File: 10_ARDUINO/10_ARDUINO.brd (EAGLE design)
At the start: 67.4 x 44.8 mm, 3 parts, among them M1 ARDUINO_PROMINI, X1 ALLSERIALSLAVE

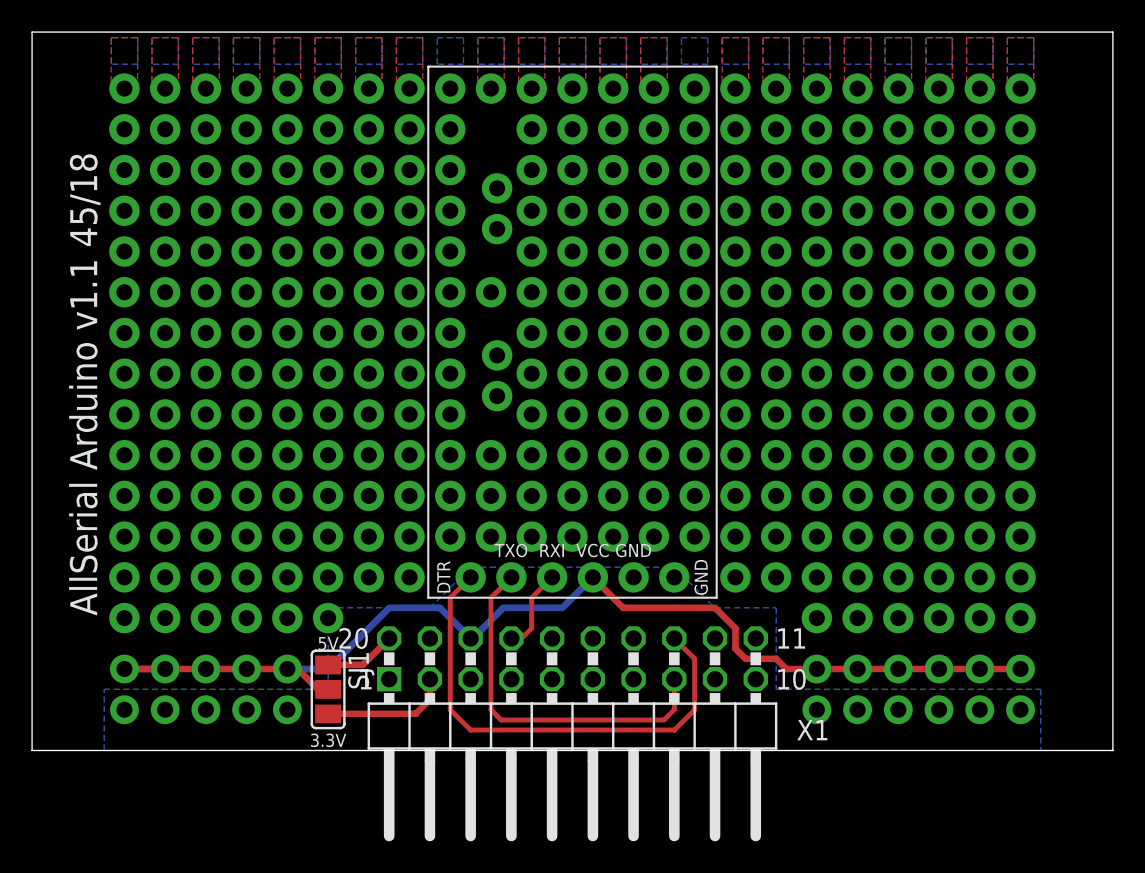
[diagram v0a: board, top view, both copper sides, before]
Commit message: Revert "pro mini layout corrected"
This reverts commit e6acf7b114fc184efa746b3a51c54623d1353390.
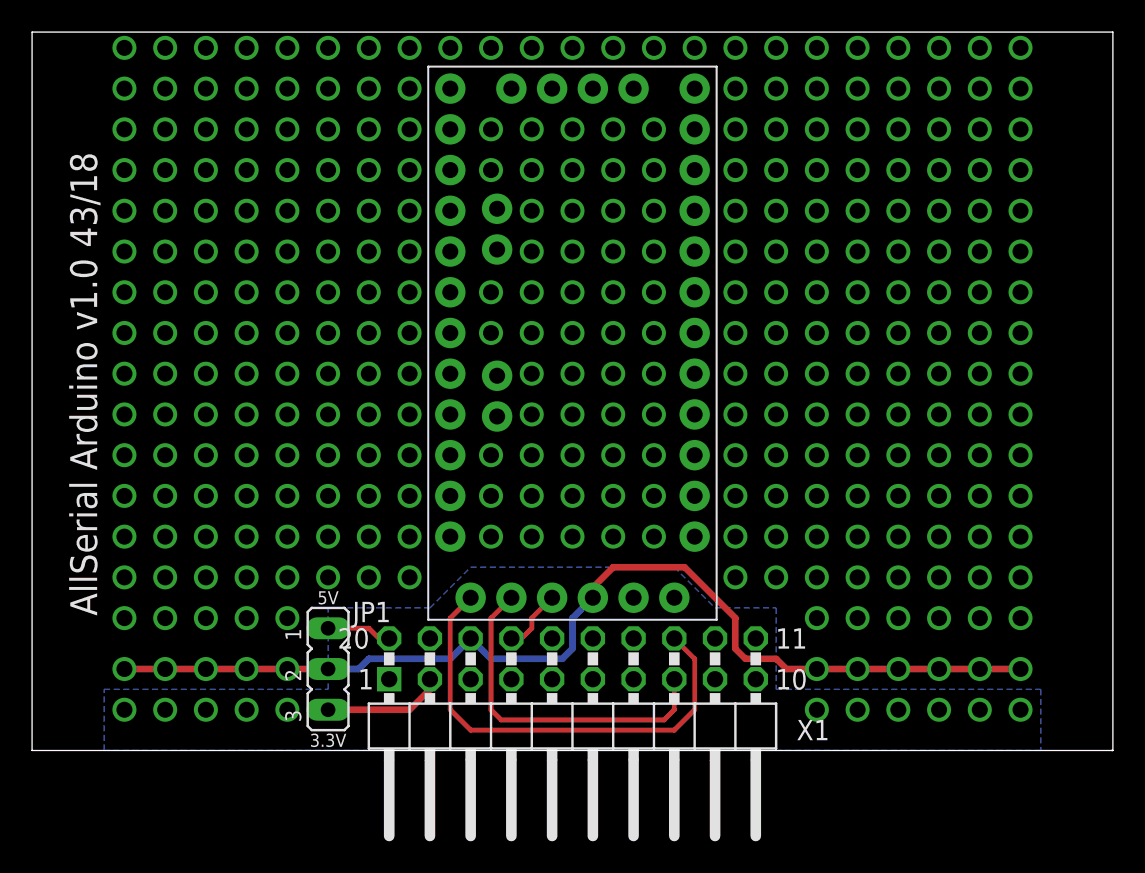
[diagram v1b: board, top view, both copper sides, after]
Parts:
- removed SJ1: (no value), jumper:SJ_2
- added JP1: (no value), jumper:JP2
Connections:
- net N$279: now also JP1.1, X1.20; no longer SJ1.3, X1.2
- net N$280: now also JP1.3, X1.2; no longer SJ1.1, X1.20
- net VCC: now also JP1.2; no longer SJ1.2
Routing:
- net N$279: track 7.99 -> 4.07 mm
- net VCC: track 68.5 -> 64.8 mm
- net N$280: track 4.49 -> 7.51 mm
- net N$2: track 22.6 -> 21.4 mm
- net N$11: track 30.0 -> 28.8 mm
- net N$1: track 5.23 -> 3.96 mm
- removed copper zone on layer 1, net N$10
- removed copper zone on layer 1, net N$100
- removed copper zone on layer 1, net N$101
- removed copper zone on layer 1, net N$102
- removed copper zone on layer 1, net N$103
- removed copper zone on layer 1, net N$104
- removed copper zone on layer 1, net N$105
- removed copper zone on layer 1, net N$106
- removed copper zone on layer 1, net N$107
- removed copper zone on layer 16, net N$245
- removed copper zone on layer 16, net N$246
- removed copper zone on layer 16, net N$247
- removed copper zone on layer 16, net N$248
- removed copper zone on layer 16, net N$249
- removed copper zone on layer 16, net N$250
- removed copper zone on layer 16, net N$251
- removed copper zone on layer 16, net N$252
- removed copper zone on layer 16, net N$253
- removed copper zone on layer 16, net N$254
- removed copper zone on layer 16, net N$255
- removed copper zone on layer 16, net N$256
- removed copper zone on layer 16, net N$257
- removed copper zone on layer 16, net N$258
- removed copper zone on layer 16, net N$259
- removed copper zone on layer 16, net N$260
- removed copper zone on layer 1, net N$276
- removed copper zone on layer 1, net N$277
- removed copper zone on layer 1, net N$278
- removed copper zone on layer 1, net N$281
- removed copper zone on layer 1, net N$282
- removed copper zone on layer 16, net N$283
- removed copper zone on layer 16, net N$284
- removed copper zone on layer 16, net N$285
- removed copper zone on layer 16, net N$286
- removed copper zone on layer 16, net N$287
- removed copper zone on layer 16, net N$288
- removed copper zone on layer 16, net N$292
- removed copper zone on layer 1, net N$3
- removed copper zone on layer 1, net N$4
- removed copper zone on layer 1, net N$5
- removed copper zone on layer 1, net N$6
- removed copper zone on layer 1, net N$7
- removed copper zone on layer 1, net N$8
- removed copper zone on layer 1, net N$9
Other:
- board text added: "AllSerial Arduino v1.0 43/18"
- board text removed: "AllSerial Arduino v1.1 45/18"
